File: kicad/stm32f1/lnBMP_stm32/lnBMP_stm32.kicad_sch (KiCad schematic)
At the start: 27 parts, among them J1 BMP Debug1, J2 BMP Debug2, J3 Debug port, J4 USB_OTG, U1 STM32F103CBTx, U2 LM1117-3.3, Y1 Crystal

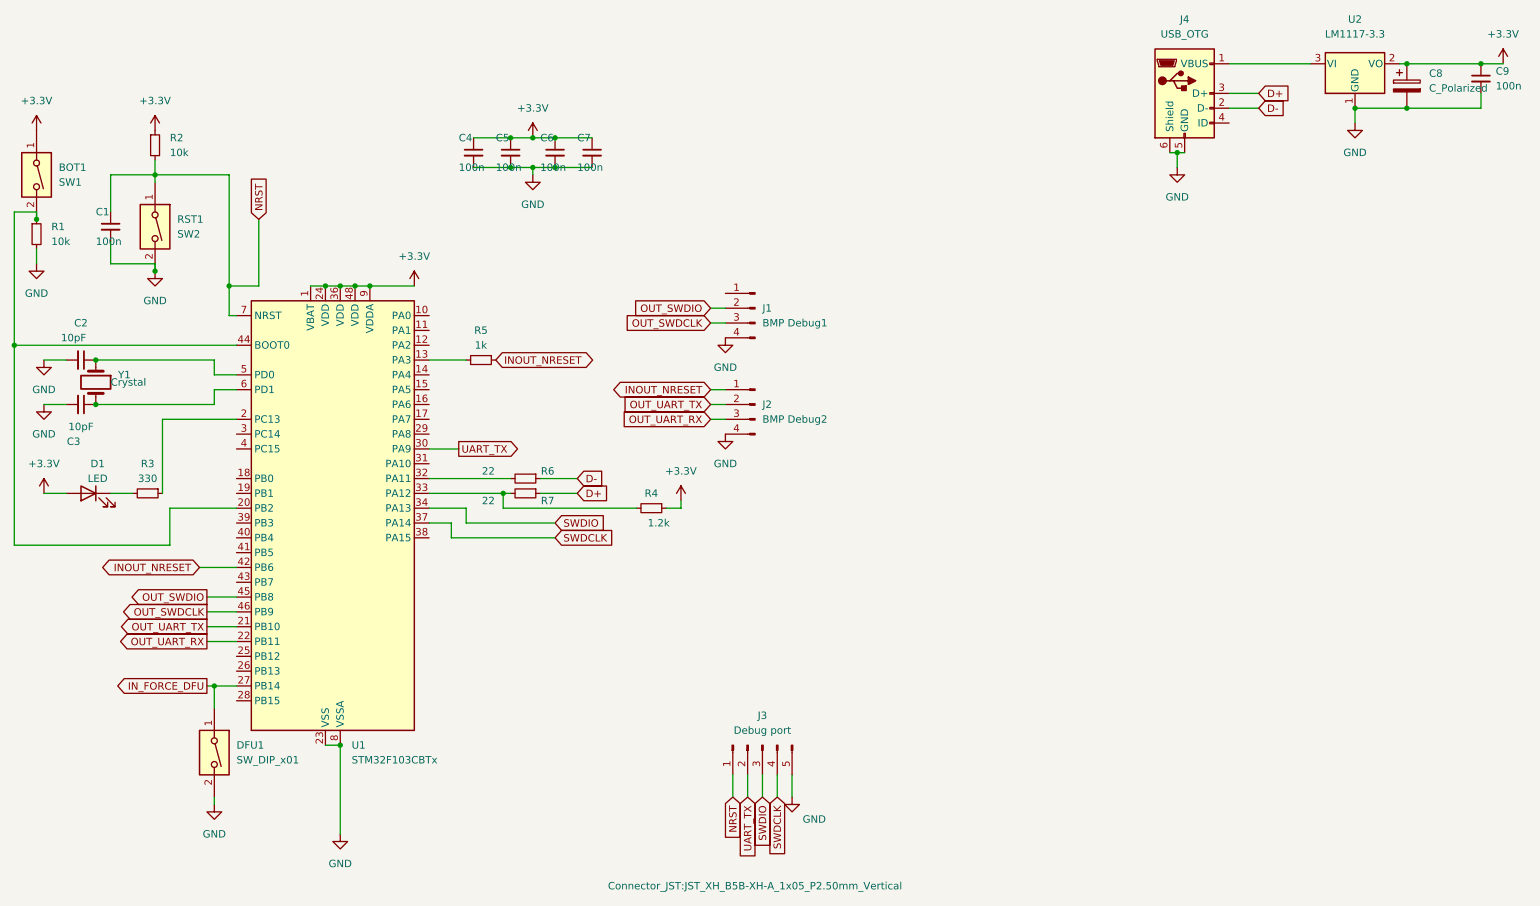
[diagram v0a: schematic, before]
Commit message: update lnArduino
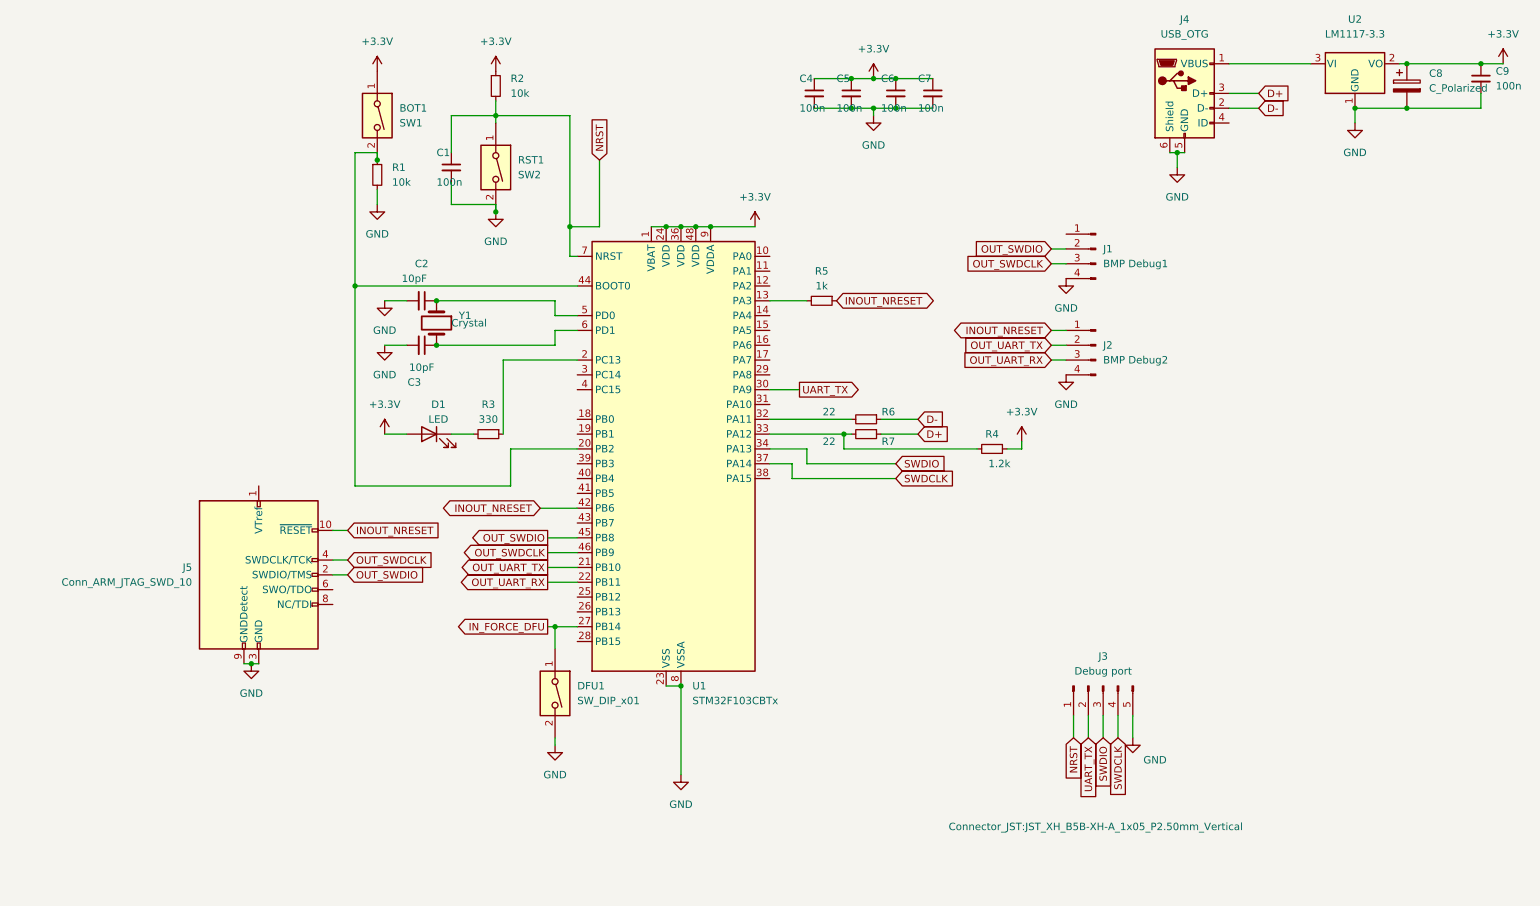
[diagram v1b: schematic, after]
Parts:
- added J5: Conn_ARM_JTAG_SWD_10, Connector_PinHeader_1.27mm:PinHeader_2x05_P1.27mm_Vertical_SMD, symbol Connector:Conn_ARM_JTAG_SWD_10
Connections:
- net GND: now also J5.3 (GND), J5.5 (GND), J5.9 (GNDDetect)
- net INOUT_NRESET: now also J5.10 (~{RESET})
- net OUT_SWDCLK: now also J5.4 (SWDCLK/TCK)
- net OUT_SWDIO: now also J5.2 (SWDIO/TMS)
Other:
- moved on the sheet: BOT1, C1, C2, C3, C4, C5, C6, C7, D1, DFU1, J1, J2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

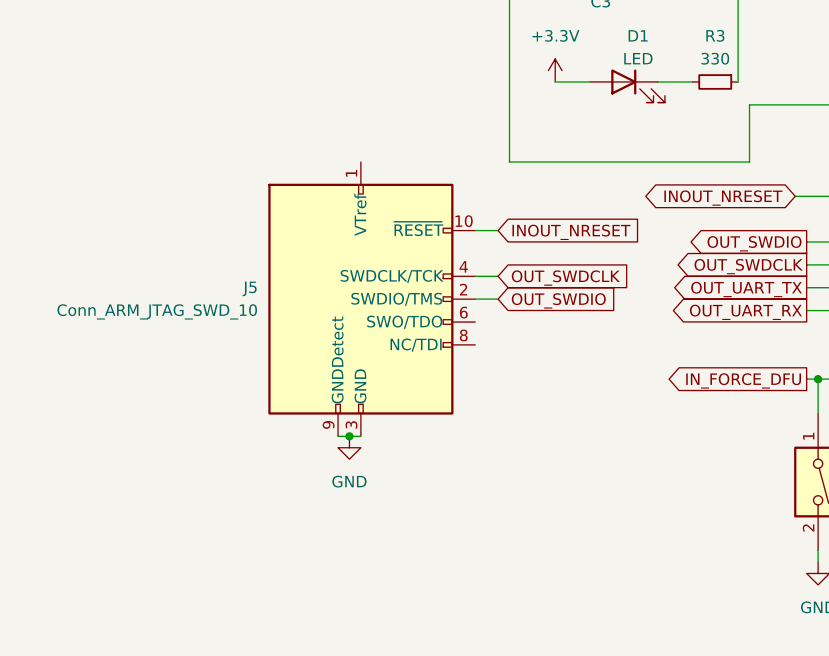
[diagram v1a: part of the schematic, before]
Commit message: cleanup kicak / stm32
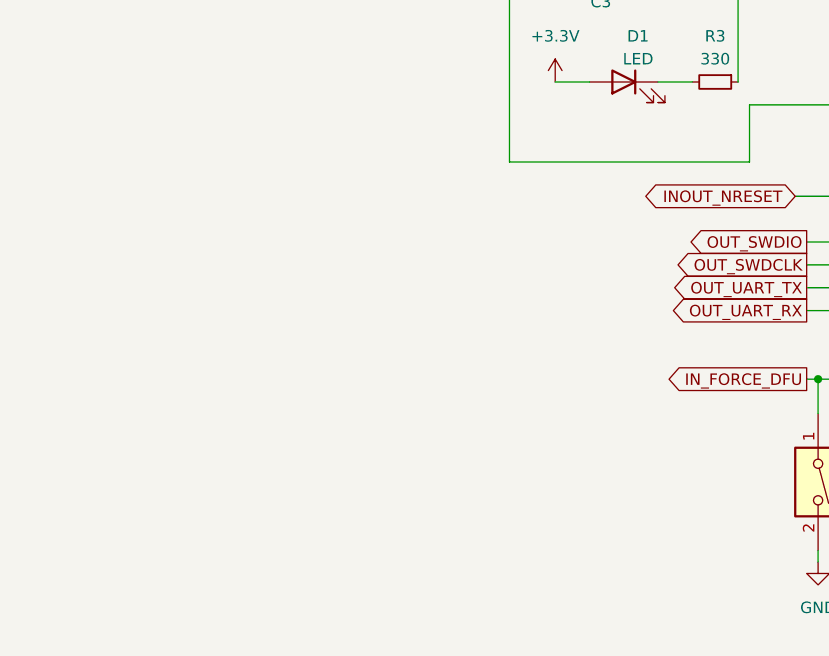
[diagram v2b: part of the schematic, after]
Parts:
- removed J5: Conn_ARM_JTAG_SWD_10, Connector_PinHeader_1.27mm:PinHeader_2x05_P1.27mm_Vertical_SMD, symbol Connector:Conn_ARM_JTAG_SWD_10
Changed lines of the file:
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@@
   (junction (at 86.36 72.39) (diameter 0) (color 0 0 0 0)
   )
-  (junction (at 54.61 127) (diameter 0) (color 0 0 0 0)
-  )
   (junction (at 157.48 26.67) (diameter 0) (color 0 0 0 0)
   )
@@
     (stroke (width 0) (type default))
   )
-  (wire (pts (xy 68.58 104.14) (xy 71.12 104.14))
-    (stroke (width 0) (type default))
-  )
   (wire (pts (xy 213.36 39.37) (xy 214.63 39.37))
     (stroke (width 0) (type default))
@@
     (stroke (width 0) (type default))
   )
-  (wire (pts (xy 53.34 127) (xy 54.61 127))
-    (stroke (width 0) (type default))
-  )
   (wire (pts (xy 109.22 52.07) (xy 109.22 57.15))
     (stroke (width 0) (type default))
@@
     (stroke (width 0) (type default))
   )
-  (wire (pts (xy 68.58 111.76) (xy 71.12 111.76))
-    (stroke (width 0) (type default))
-  )
   (wire (pts (xy 72.39 62.23) (xy 110.49 62.23))
     (stroke (width 0) (type default))
@@
     (stroke (width 0) (type default))
   )
-  (wire (pts (xy 54.61 127) (xy 55.88 127))
-    (stroke (width 0) (type default))
-  )
   (wire (pts (xy 72.39 39.37) (xy 76.2 39.37))
     (stroke (width 0) (type default))
@@
   )
   (wire (pts (xy 143.51 85.09) (xy 157.48 85.09))
-    (stroke (width 0) (type default))
-  )
-  (wire (pts (xy 68.58 109.22) (xy 71.12 109.22))
     (stroke (width 0) (type default))
   )
@@
     )
   )
-  (global_label "OUT_SWDIO" (shape input) (at 71.12 111.76 0) (fields_autoplaced)
-    (effects (font (size 1.27 1.27)) (justify left))
-    (property "Intersheetrefs" "${INTERSHEET_REFS}" (at 84.5676 111.76 0)
-      (effects (font (size 1.27 1.27)) (justify left) hide)
-    )
-  )
   (global_label "D-" (shape input) (at 168.91 85.09 0) (fields_autoplaced)
     (effects (font (size 1.27 1.27)) (justify left))
@@
     )
   )
-  (global_label "INOUT_NRESET" (shape input) (at 71.12 104.14 0) (fields_autoplaced)
-    (effects (font (size 1.27 1.27)) (justify left))
-    (property "Intersheetrefs" "${INTERSHEET_REFS}" (at 87.7123 104.14 0)
-      (effects (font (size 1.27 1.27)) (justify left) hide)
-    )
-  )
   (global_label "OUT_UART_RX" (shape input) (at 191.77 74.93 180) (fields_autoplaced)
     (effects (font (size 1.27 1.27)) (justify right))
@@
     )
   )
-  (global_label "OUT_SWDCLK" (shape input) (at 71.12 109.22 0) (fields_autoplaced)
-    (effects (font (size 1.27 1.27)) (justify left))
-    (property "Intersheetrefs" "${INTERSHEET_REFS}" (at 86.2004 109.22 0)
-      (effects (font (size 1.27 1.27)) (justify left) hide)
-    )
-  )
   (global_label "INOUT_NRESET" (shape bidirectional) (at 104.14 100.33 180) (fields_autoplaced)
     (effects (font (size 1.27 1.27)) (justify right))
@@
     )
   )
-  (symbol (lib_id "power:GND") (at 54.61 127 0) (unit 1)
-    (exclude_from_sim no) (in_bom yes) (on_board yes) (dnp no) (fields_autoplaced)
-    (property "Reference" "#PWR04" (at 54.61 133.35 0)
-      (effects (font (size 1.27 1.27)) hide)
-    )
-    (property "Value" "GND" (at 54.61 132.08 0)
-      (effects (font (size 1.27 1.27)))
-    )
-    (property "Footprint" "" (at 54.61 127 0)
-      (effects (font (size 1.27 1.27)) hide)
-    )
-    (property "Datasheet" "" (at 54.61 127 0)
-      (effects (font (size 1.27 1.27)) hide)
-    )
-    (property "Description" "" (at 54.61 127 0)
-      (effects (font (size 1.27 1.27)) hide)
-    )
-    (pin "1")
-    (instances
-      (project "lnBMP_stm32"
-        (path "/fbe443d6-6d74-4abc-9dee-16e0160553bc"
-          (reference "#PWR04") (unit 1)
-        )
-      )
-    )
-  )
   (symbol (lib_id "Device:C_Small") (at 165.1 29.21 0) (unit 1)
     (exclude_from_sim no) (in_bom yes) (on_board yes) (dnp no)
@@
         )
       )
-    )
-  )
-  (symbol (lib_id "Connector:Conn_ARM_JTAG_SWD_10") (at 55.88 111.76 0) (unit 1)
-    (exclude_from_sim no) (in_bom yes) (on_board yes) (dnp no) (fields_autoplaced)
-    (property "Reference" "J5" (at 44.45 110.4899 0)
-      (effects (font (size 1.27 1.27)) (justify right))
-    )
-    (property "Value" "Conn_ARM_JTAG_SWD_10" (at 44.45 113.0299 0)
-      (effects (font (size 1.27 1.27)) (justify right))
-    )
-    (property "Footprint" "Connector_PinHeader_1.27mm:PinHeader_2x05_P1.27mm_Vertical_SMD" (at 55.88 111.76 0)
-      (effects (font (size 1.27 1.27)) hide)
-    )
-    (property "Datasheet" "http://infocenter.arm.com/help/topic/com.arm.doc.ddi0314h/DDI0314H_coresight_components_trm.pdf" (at 46.99 143.51 90)
-      (effects (font (size 1.27 1.27)) hide)
-    )
-    (property "Description" "Cortex Debug Connector, standard ARM Cortex-M SWD and JTAG interface" (at 55.88 111.76 0)
-      (effects (font (size 1.27 1.27)) hide)
-    )
-    (pin "8")
-    (pin "7")
-    (pin "9")
-    (pin "4")
-    (pin "5")
-    (pin "1")
-    (pin "6")
-    (pin "2")
-    (pin "10")
-    (pin "3")
-    (instances
-      (project "lnBMP_stm32"
-        (path "/fbe443d6-6d74-4abc-9dee-16e0160553bc"
-          (reference "J5") (unit 1)
-        )
-      )
